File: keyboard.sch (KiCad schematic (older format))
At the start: 17 parts, among them P1 USB_C_Plug_USB2.0, SW1 SW_Push, U1 ATmega32U4-AU, Y1 16MHz

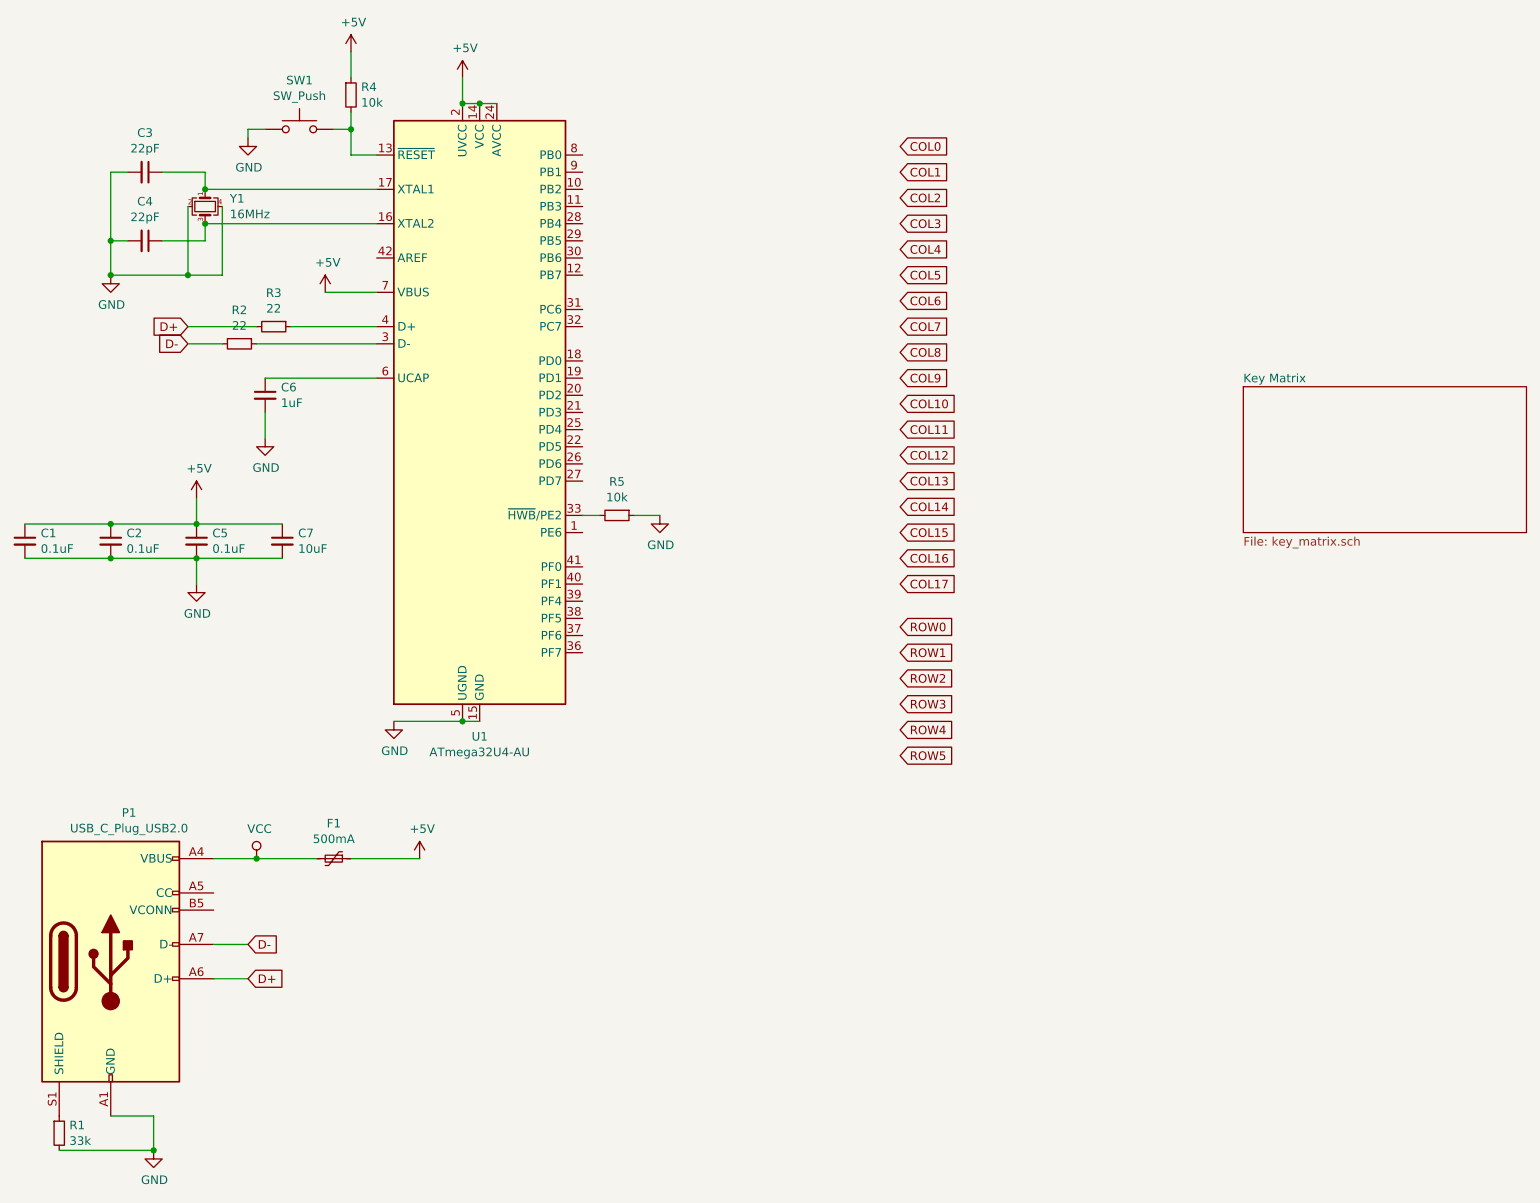
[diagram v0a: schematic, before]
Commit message: Routing & LEDS
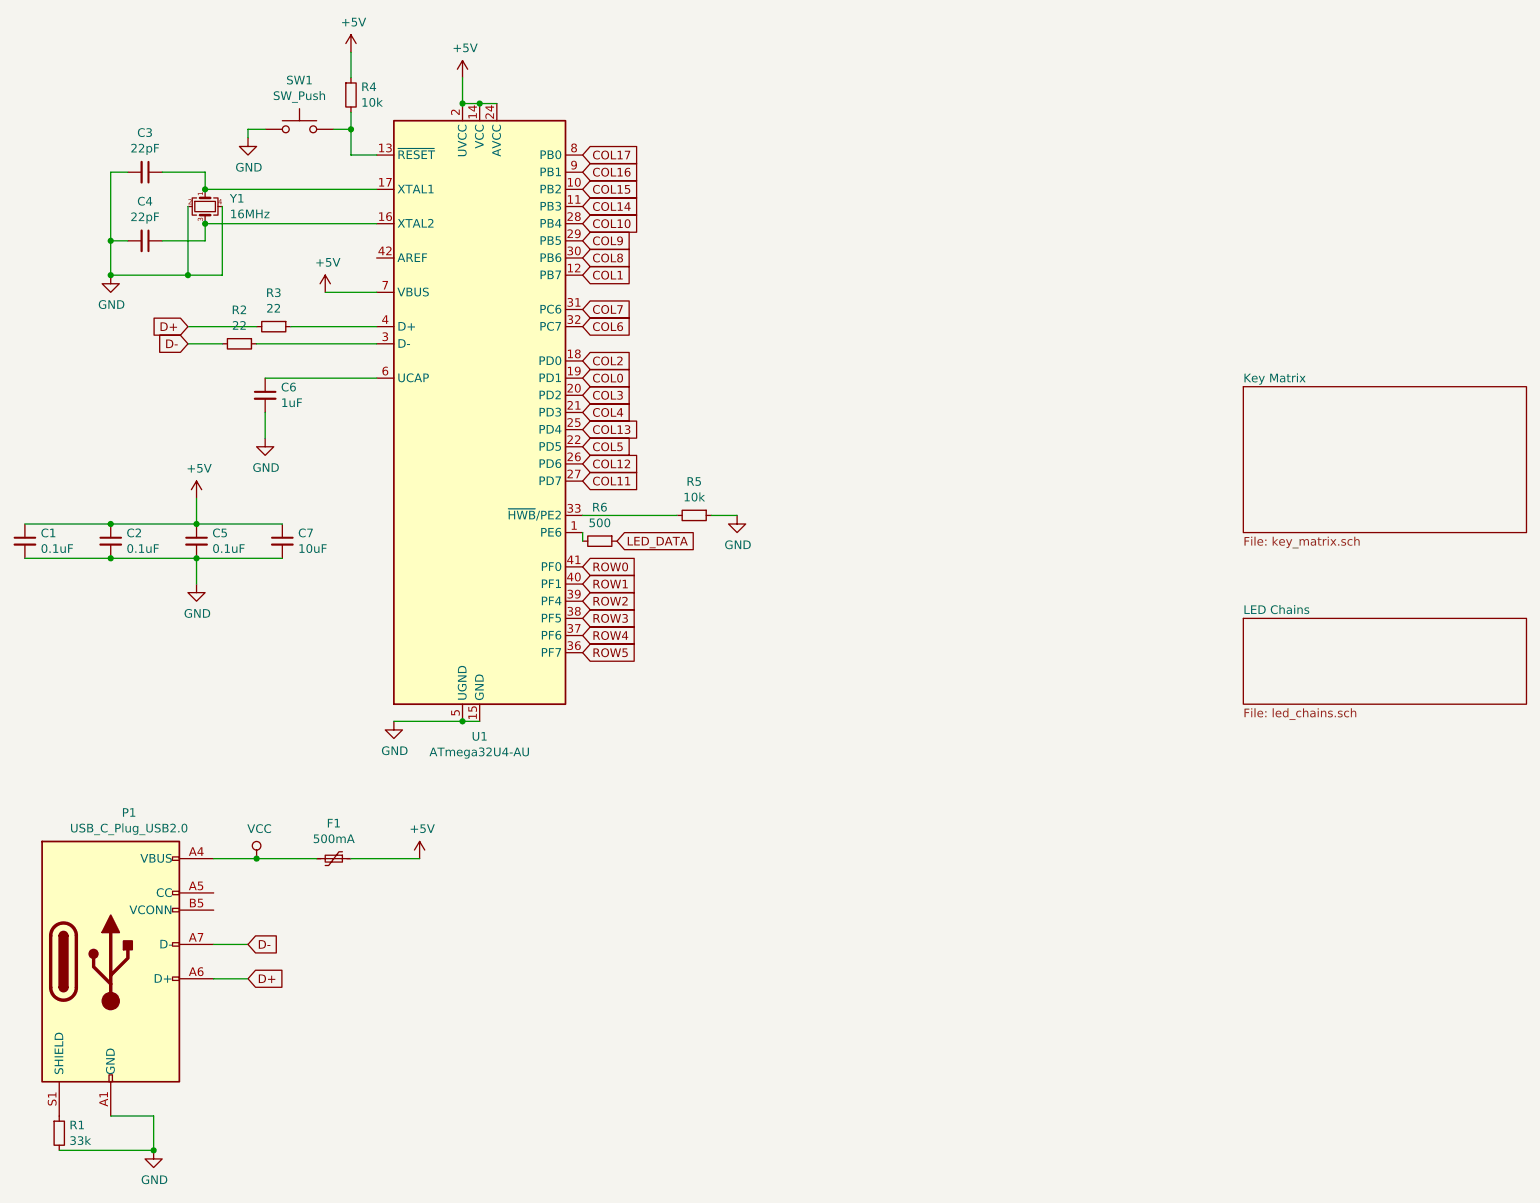
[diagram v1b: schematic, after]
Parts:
- added R6: 500, Resistor_SMD:R_0805_2012Metric, symbol Device:R_Small
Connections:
- net COL0: now also U1.19 (PD1)
- net COL1: now also U1.12 (PB7)
- net COL10: now also U1.28 (PB4)
- net COL11: now also U1.27 (PD7)
- net COL12: now also U1.26 (PD6)
- net COL13: now also U1.25 (PD4)
- net COL14: now also U1.11 (PB3)
- net COL15: now also U1.10 (PB2)
- net COL16: now also U1.9 (PB1)
- net COL17: now also U1.8 (PB0)
- net COL2: now also U1.18 (PD0)
- net COL3: now also U1.20 (PD2)
- net COL4: now also U1.21 (PD3)
- net COL5: now also U1.22 (PD5)
- net COL6: now also U1.32 (PC7)
- net COL7: now also U1.31 (PC6)
- net COL8: now also U1.30 (PB6)
- net COL9: now also U1.29 (PB5)
- net ROW0: now also U1.41 (PF0)
- net ROW1: now also U1.40 (PF1)
- net ROW2: now also U1.39 (PF4)
- net ROW3: now also U1.38 (PF5)
- net ROW4: now also U1.37 (PF6)
- net ROW5: now also U1.36 (PF7)
- net at U1.1 (PE6): now also R6.2
- new net LED_DATA: R6.1
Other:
- moved on the sheet: R5
